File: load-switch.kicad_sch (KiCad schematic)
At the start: 14 parts, among them IC3 TPS2H160AQPWPRQ1, IC4 TPS2H160AQPWPRQ1

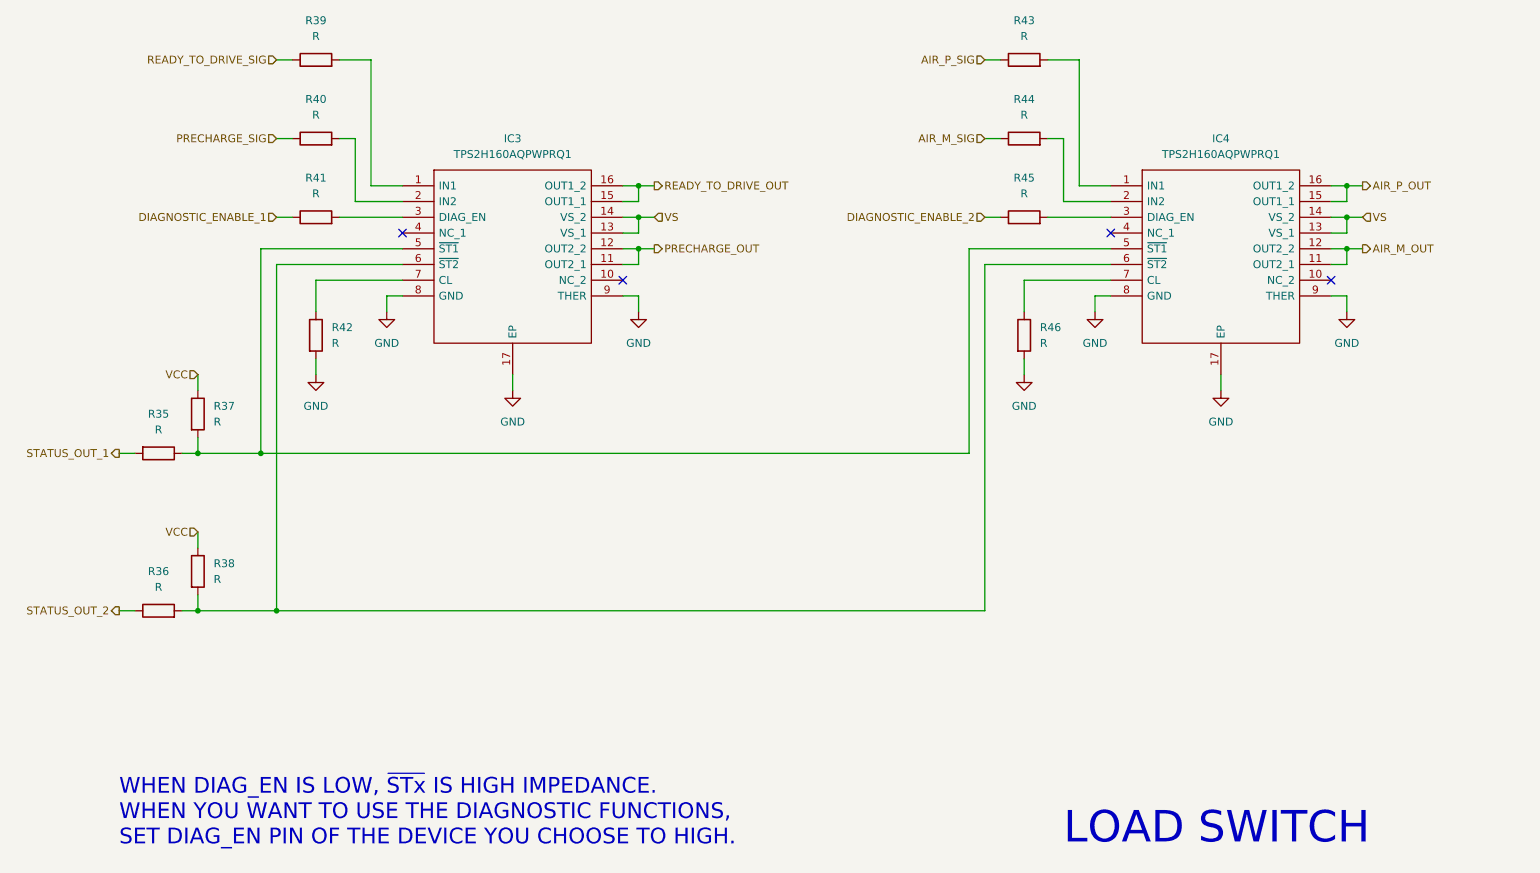
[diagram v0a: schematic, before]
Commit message: decide constant, modify
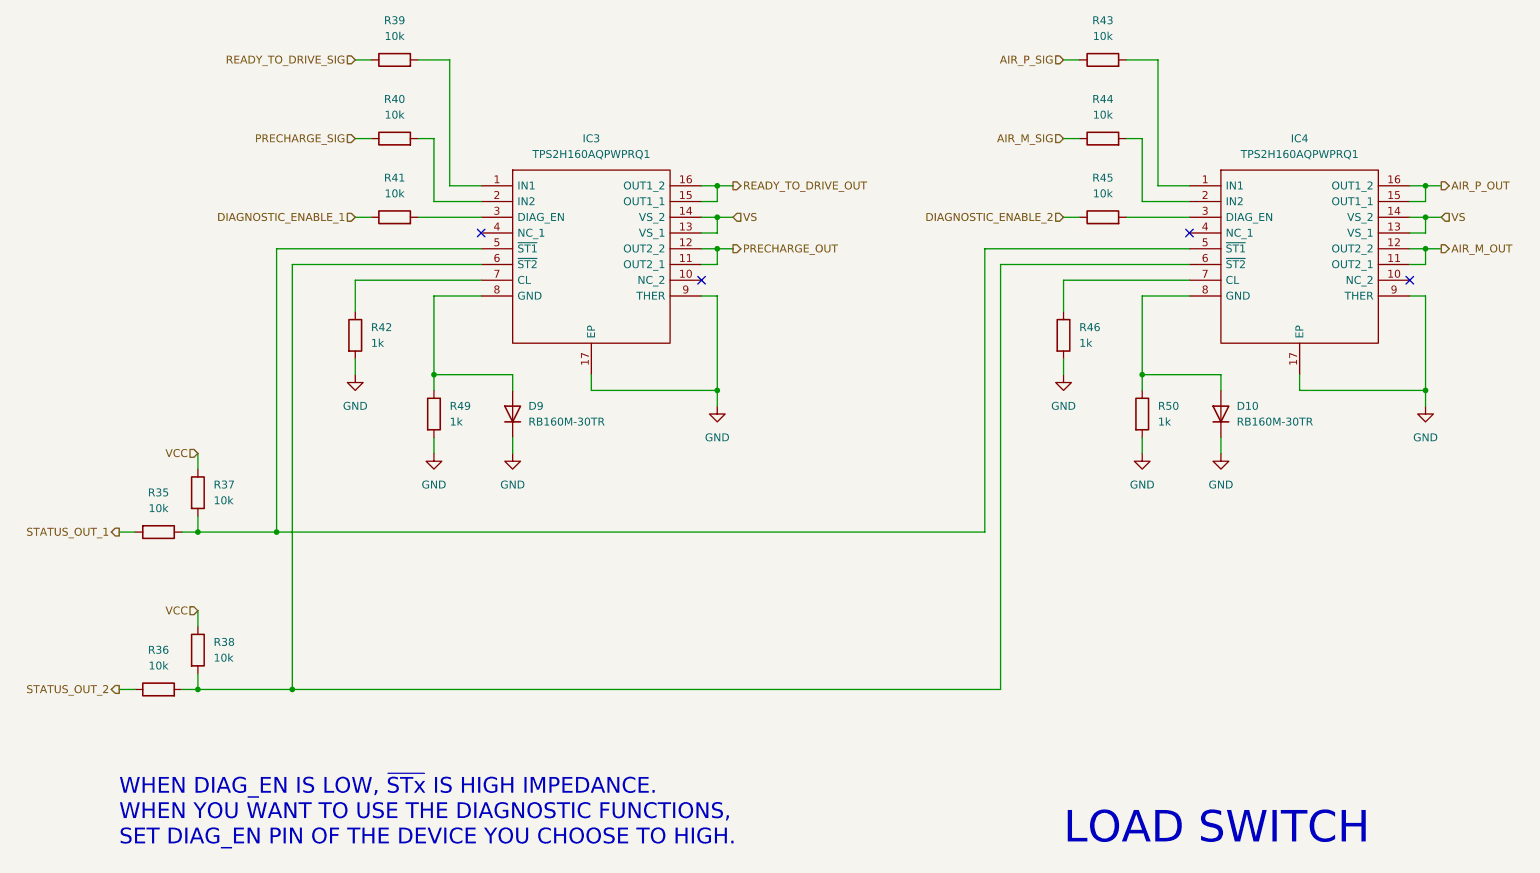
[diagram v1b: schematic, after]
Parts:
- added D10, D9: RB160M-30TR, Diode_SMD:D_SOD-123F, symbol Device:D
- added R49, R50: 1k, symbol Device:R
- R35, R36, R37, R38, R39, R40, R41, R43, R44, R45: value R -> 10k
- R42, R46: value R -> 1k
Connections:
- net GND: now also D10.1 (K), D9.1 (K), R49.2, R50.2; no longer IC3.8 (GND), IC4.8 (GND)
- new net: D9.2 (A), IC3.8 (GND), R49.1
- new net: D10.2 (A), IC4.8 (GND), R50.1
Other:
- moved on the sheet: IC3, IC4, R35, R36, R37, R38, R39, R40, R41, R42, R43, R44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
